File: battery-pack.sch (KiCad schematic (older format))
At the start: 54 parts, among them P1 CONN_01X02, U1 18650-PC8, U2 18650-PC8, U3 18650-PC8, U4 18650-PC8

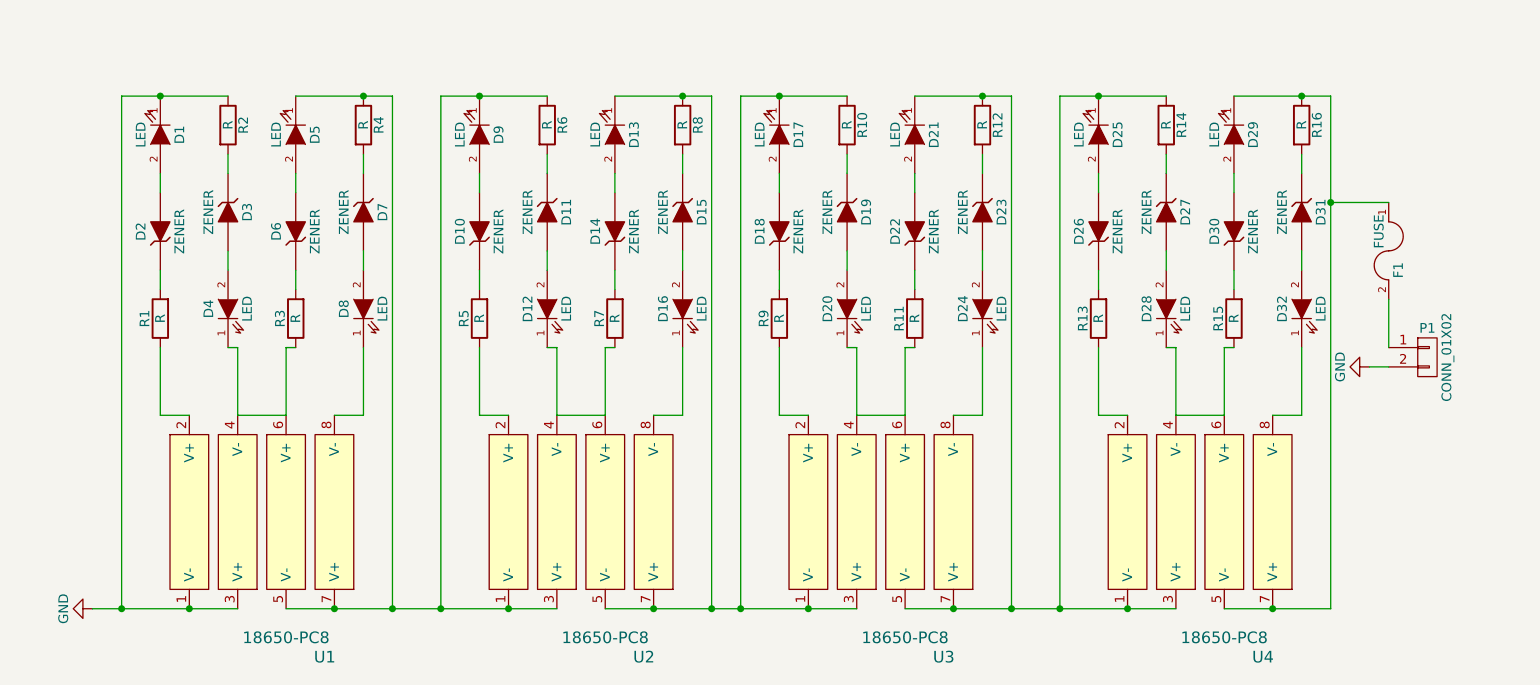
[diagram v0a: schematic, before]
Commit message: updated schematic
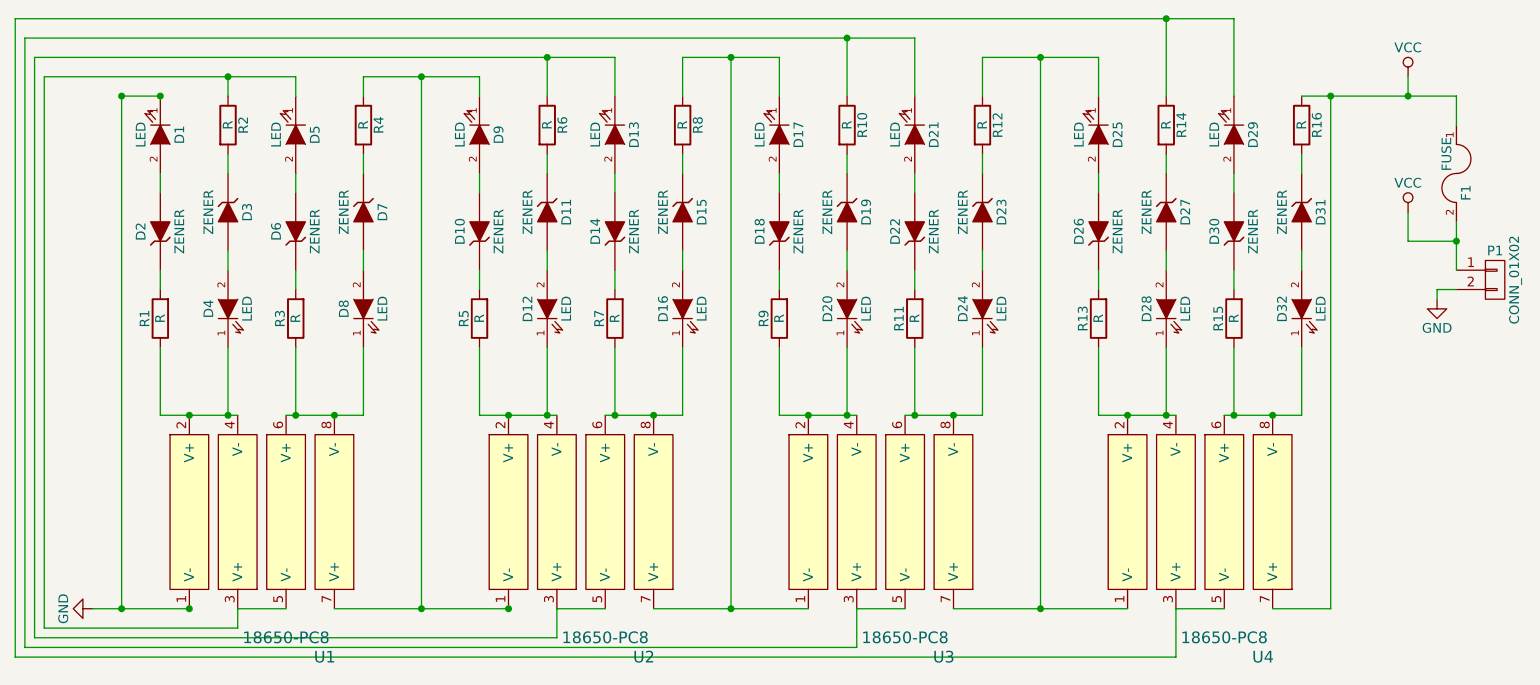
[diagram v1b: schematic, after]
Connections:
- net GND: no longer R2.1, U1.3 (V+)
- net at R1.1, U1.2 (V+): now also D4.1 (K), U1.4 (V-)
- net at R3.1, U1.6 (V+): now also D8.1 (K), U1.8 (V-); no longer D4.1 (K), U1.4 (V-)
- net at D9.1 (K), R4.1, U1.7 (V+)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: no longer D5.1 (K), R6.1, U1.5 (V-), U2.3 (V+)
- net at R5.1, U2.2 (V+): now also D12.1 (K), U2.4 (V-)
- net at R7.1, U2.6 (V+): now also D16.1 (K), U2.8 (V-); no longer D12.1 (K), U2.4 (V-)
- net at D17.1 (K), R8.1, U2.7 (V+)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: no longer D13.1 (K), R10.1, U2.5 (V-), U3.3 (V+)
- net at R9.1, U3.2 (V+): now also D20.1 (K), U3.4 (V-)
- net at R11.1, U3.6 (V+): now also D24.1 (K), U3.8 (V-); no longer D20.1 (K), U3.4 (V-)
- net at D25.1 (K), R12.1, U3.7 (V+)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: no longer D21.1 (K), R14.1, U3.5 (V-), U4.3 (V+)
- net at R13.1, U4.2 (V+): now also D28.1 (K), U4.4 (V-)
- net at R15.1, U4.6 (V+): now also D32.1 (K), U4.8 (V-); no longer D28.1 (K), U4.4 (V-)
- net VCC: now reaches F1.1, R16.1, U4.7 (V+)
- net VCC: now also F1.2, P1.1 (P1); no longer D29.1 (K), U4.5 (V-)
- new net: D5.1 (K), R2.1, U1.3 (V+), U1.5 (V-)
- new net: D13.1 (K), R6.1, U2.3 (V+), U2.5 (V-)
- new net: D21.1 (K), R10.1, U3.3 (V+), U3.5 (V-)
- new net: D29.1 (K), R14.1, U4.3 (V+), U4.5 (V-)
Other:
- moved on the sheet: F1, P1

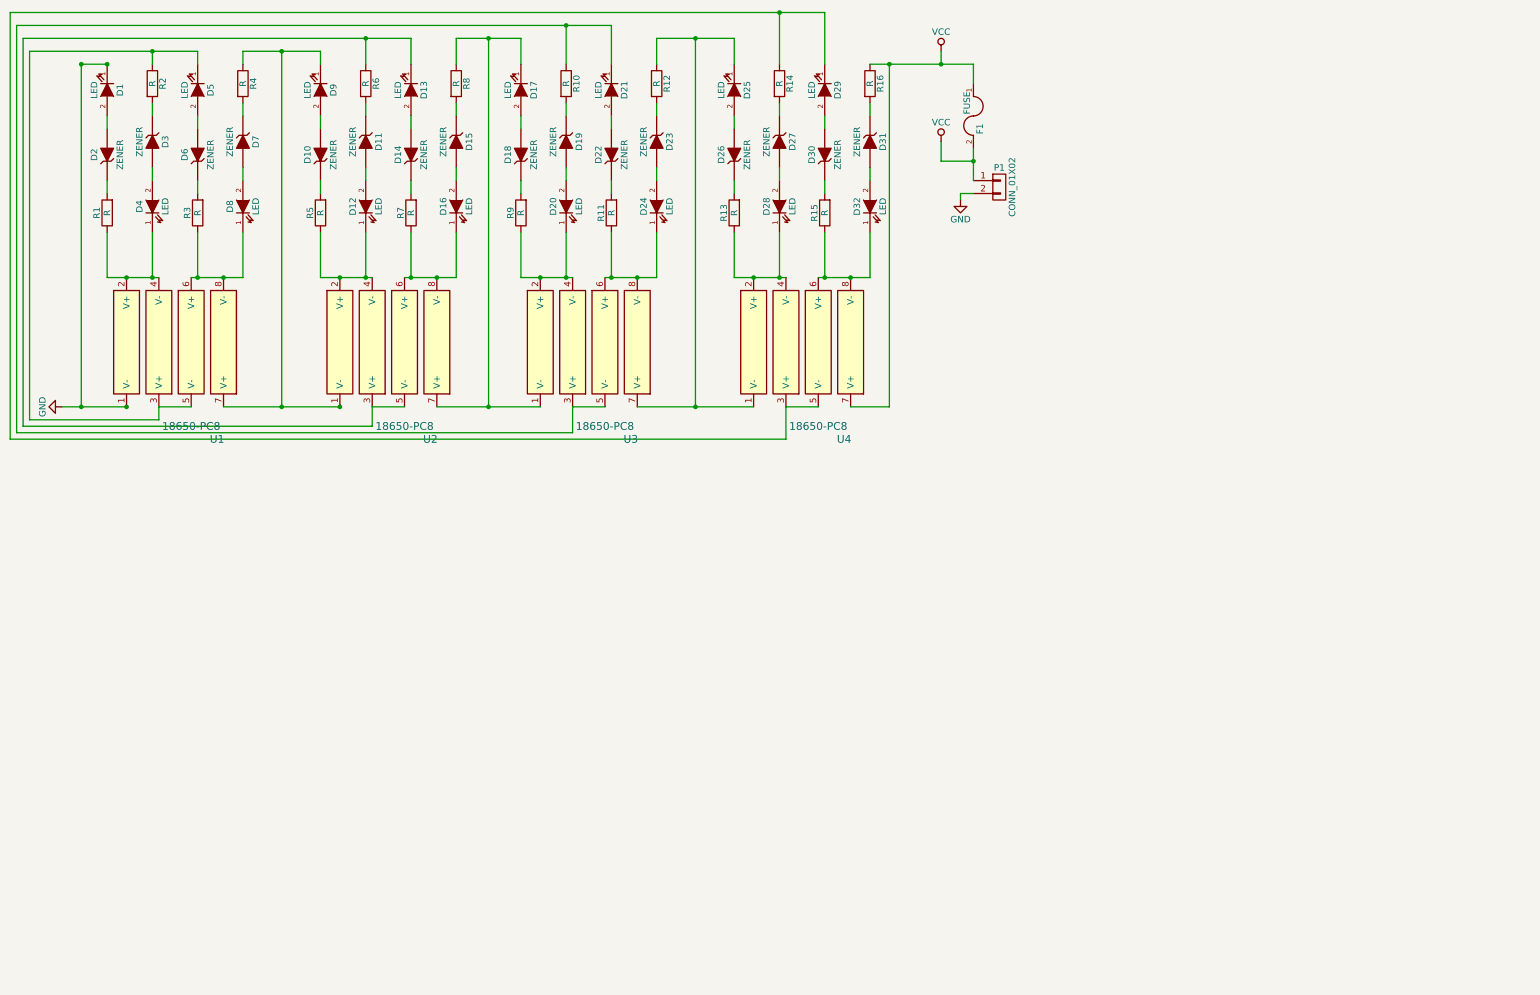
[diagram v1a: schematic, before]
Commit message: update
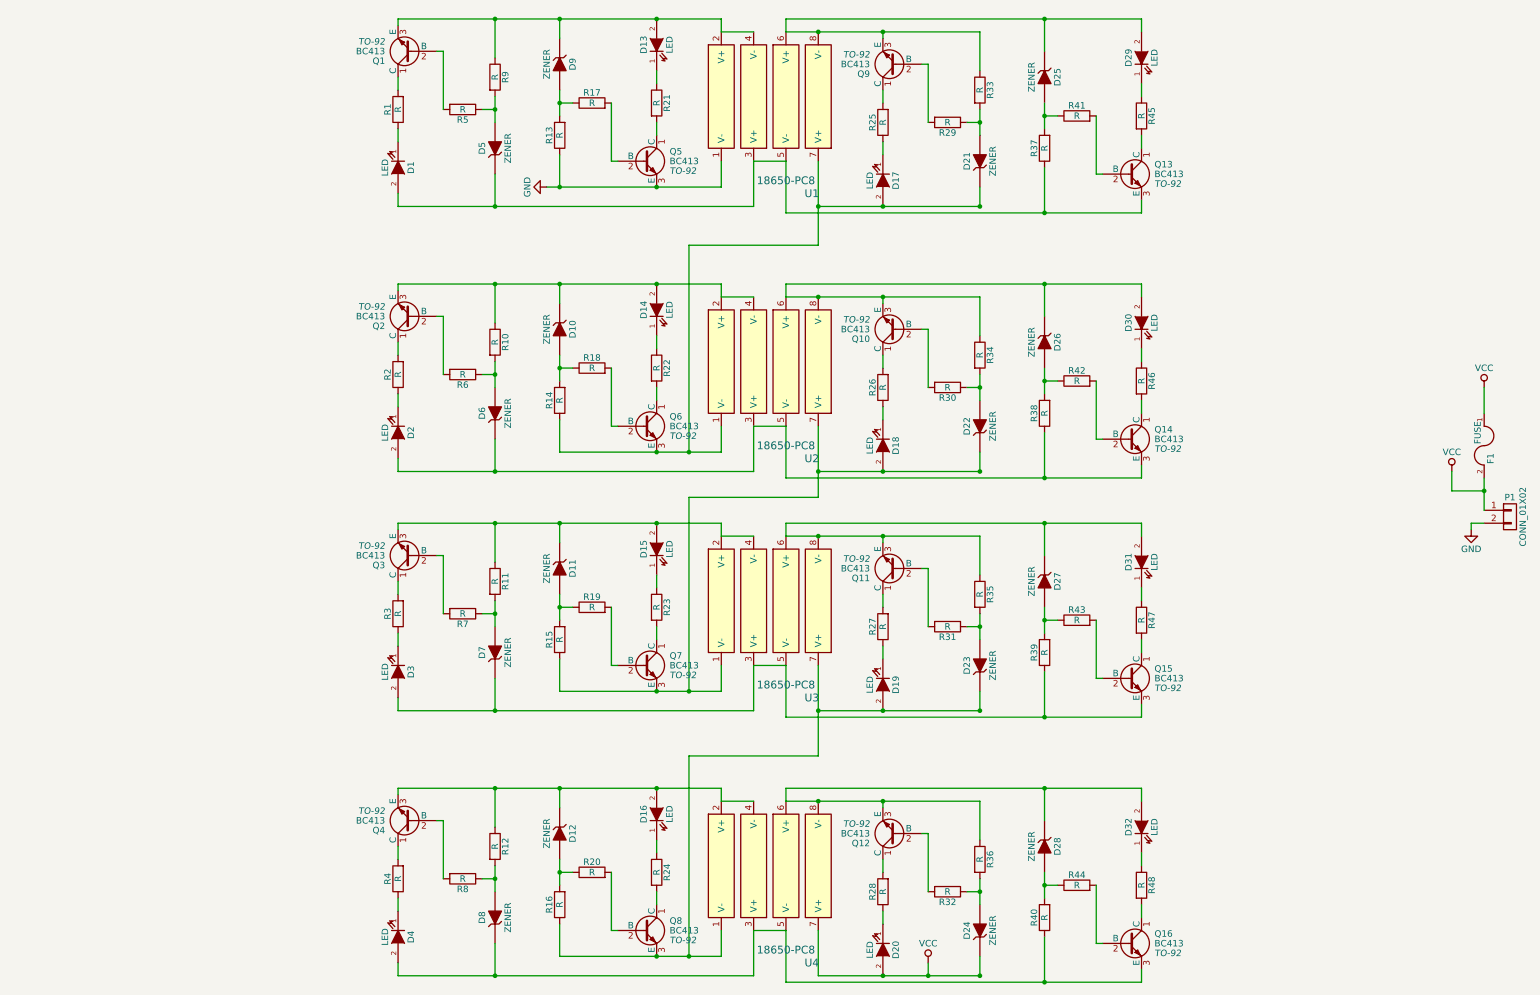
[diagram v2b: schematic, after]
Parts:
- removed D12, D21, D24, D25, D28, D5, D8, D9: LED, LEDs:LED-1206, symbol LED
- removed D14, D15, D18, D19, D2, D3, D30, D31: ZENER, LEDs:LED-1206, symbol ZENER
- added D12, D21, D24, D25, D28, D5, D8, D9: ZENER, LEDs:LED-1206, symbol ZENER
- added D14, D15, D18, D19, D2, D3, D30, D31: LED, LEDs:LED-1206, symbol LED
- added Q1, Q10, Q11, Q12, Q13, Q14, Q15, Q16, Q2, Q3, Q4, Q5, Q6, Q7, Q8, Q9: BC413, TO-92, symbol BC413
- added R17, R18, R19, R20, R21, R22, R23, R24, R25, R26, R27, R28, R29, R30, R31, R32, R33, R34, R35, R36, R37, R38, R39, R40, R41, R42, R43, R44, R45, R46, R47, R48: R, Resistors_SMD:R_1206, symbol R
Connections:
- net GND: now also R13.1, Q5.3 (E); no longer D1.1 (K)
- net VCC: now also D20.2 (A), D24.1 (K); no longer R16.1
- net at U1.2 (V+), U1.4 (V-): now also D13.2 (A), R9.1, D9.1 (K), Q1.3 (E); no longer D4.1 (K), R1.1
- net at U1.3 (V+), U1.5 (V-): now also D1.2 (A), D5.1 (K), Q13.3 (E), R37.1; no longer R2.1
- net at U1.6 (V+), U1.8 (V-): now also D29.2 (A), D25.1 (K), Q9.3 (E), R33.1; no longer R3.1
- net at U1.7 (V+), U2.1 (V-): now also D17.2 (A), R14.1, D21.1 (K), Q6.3 (E); no longer R4.1
- net at D4.2 (A): now also U4.3 (V+), U4.5 (V-), D8.1 (K), Q16.3 (E), R40.1
- net at R2.2: now also Q2.1 (C)
- net at R1.2: now also Q1.1 (C)
- net at D7.2 (A): now also R11.2, R7.1
- net at D7.1 (K): now also U3.3 (V+), U3.5 (V-), D3.2 (A), Q15.3 (E), R39.1; no longer R4.2
- net at D6.2 (A): now also R10.2, R6.1
- net at R3.2: now also Q3.1 (C); no longer D6.1 (K)
- net at U2.2 (V+), U2.4 (V-): now also D10.1 (K), R10.1, D14.2 (A), Q2.3 (E); no longer R5.1
- net at U2.3 (V+), U2.5 (V-): now also D6.1 (K), D2.2 (A), Q14.3 (E), R38.1; no longer D13.1 (K), R6.1
- net at U2.6 (V+), U2.8 (V-): now also D26.1 (K), D30.2 (A), Q10.3 (E), R34.1; no longer D16.1 (K), R7.1
- net at U2.7 (V+), U3.1 (V-): now also D22.1 (K), R15.1, D18.2 (A), Q7.3 (E); no longer D17.1 (K), R8.1
- net at D11.2 (A): now also R15.2, R19.1
- net at D11.1 (K): now also R11.1, U3.2 (V+), U3.4 (V-), D15.2 (A), Q3.3 (E); no longer R6.2
- net at D10.2 (A): now also R14.2, R18.1
- net at R5.2: now also Q1.2 (B); no longer D10.1 (K)
- net at D16.2 (A): now also R12.1, U4.2 (V+), U4.4 (V-), D12.1 (K), Q4.3 (E)
- net at R8.2: now also Q4.2 (B)
- net at R7.2: now also Q3.2 (B)
- net at U3.6 (V+), U3.8 (V-): now also D27.1 (K), D31.2 (A), Q11.3 (E), R35.1; no longer R11.1
- net at U3.7 (V+), U4.1 (V-): now also D23.1 (K), R16.1, D19.2 (A), Q8.3 (E); no longer R12.1
- net at R9.2: now also R5.1, D5.2 (A)
- net at D23.2 (A): now also R31.1, R35.2
- net at R12.2: now also R8.1, D8.2 (A); no longer D23.1 (K)
- net at D22.2 (A): now also R30.1, R34.2
- net at U4.6 (V+), U4.8 (V-): now also D32.2 (A), D28.1 (K), Q12.3 (E), R36.1; no longer D32.1 (K), R15.1
- net at D27.2 (A): now also R39.2, R43.1
- net at D26.2 (A): now also R38.2, R42.1
- net at R13.2: now also D9.2 (A), R17.1; no longer D26.1 (K)
- net at R16.2: now also D12.2 (A), R20.1
- new net: Q7.1 (C), R23.2
- new net: Q7.2 (B), R19.2
- new net: D15.1 (K), R23.1
- new net: D3.1 (K), R3.1
- new net: Q11.1 (C), R27.2
- new net: Q11.2 (B), R31.2
- new net: D19.1 (K), R27.1
- new net: Q15.1 (C), R47.2
- new net: Q15.2 (B), R43.2
- new net: D31.1 (K), R47.1
- new net: Q8.1 (C), R24.2
- new net: Q8.2 (B), R20.2
- new net: D16.1 (K), R24.1
- new net: Q4.1 (C), R4.2
- new net: D4.1 (K), R4.1
- new net: D24.2 (A), R32.1, R36.2
- new net: Q12.1 (C), R28.2
- new net: Q12.2 (B), R32.2
- new net: D20.1 (K), R28.1
- new net: D28.2 (A), R40.2, R44.1
- new net: Q16.1 (C), R48.2
- new net: Q16.2 (B), R44.2
- new net: D32.1 (K), R48.1
- new net: Q5.1 (C), R21.2
- new net: Q5.2 (B), R17.2
- new net: D13.1 (K), R21.1
- new net: D1.1 (K), R1.1
- new net: D21.2 (A), R29.1, R33.2
- new net: Q9.1 (C), R25.2
- new net: Q9.2 (B), R29.2
- new net: D17.1 (K), R25.1
- new net: D25.2 (A), R37.2, R41.1
- new net: Q13.1 (C), R45.2
- new net: Q13.2 (B), R41.2
- new net: D29.1 (K), R45.1
- new net: Q6.1 (C), R22.2
- new net: Q6.2 (B), R18.2
- new net: D14.1 (K), R22.1
- new net: Q2.2 (B), R6.2
- new net: D2.1 (K), R2.1
- new net: Q10.1 (C), R26.2
- new net: Q10.2 (B), R30.2
- new net: D18.1 (K), R26.1
- new net: Q14.1 (C), R46.2
- new net: Q14.2 (B), R42.2
- new net: D30.1 (K), R46.1
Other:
- moved on the sheet: F1, P1

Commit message: update
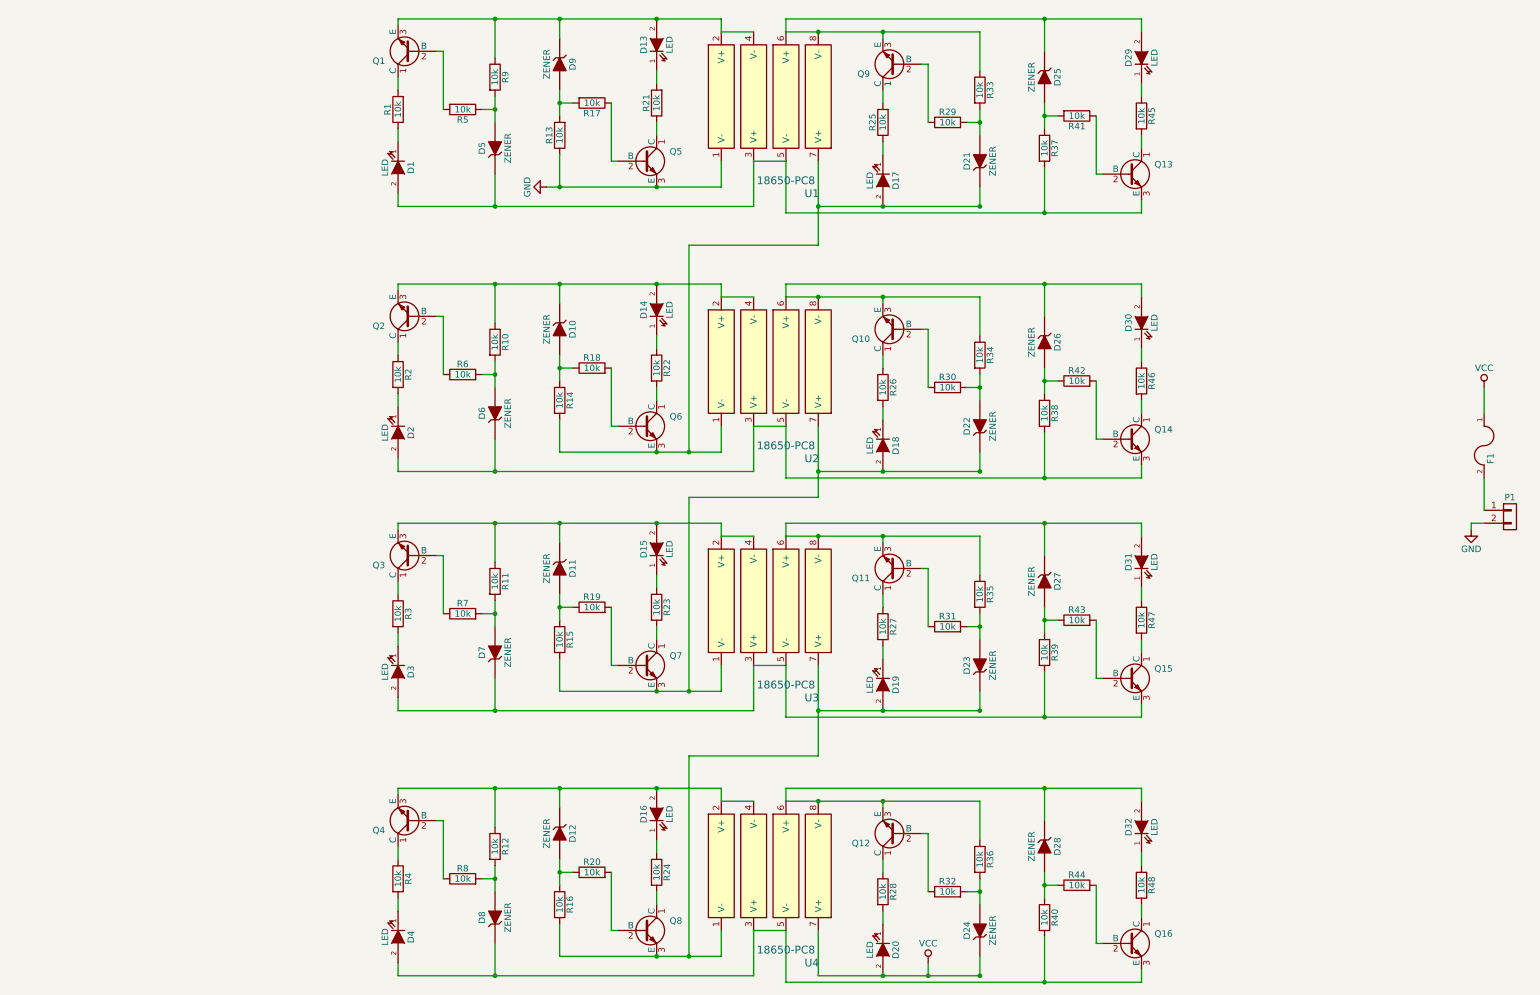
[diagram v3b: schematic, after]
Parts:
- D1, D13, D14, D15, D16, D17, D18, D19, D2, D20, D29, D3, D30, D31, D32, D4: footprint LEDs:LED-1206 -> LEDs:LED_0805
- D10, D11, D12, D21, D22, D23, D24, D25, D26, D27, D28, D6, D7, D8, D9: footprint LEDs:LED-1206 -> TO_SOT_Packages_SMD:SOT-23
- D5: footprint LEDs:LED-1206 -> Diodes_ThroughHole:Diode_P600_Horizontal
- F1: value FUSE -> 01000057Z; footprint battery-pack:fuse-holder-BK6010 -> battery-pack:ATC_FUSE
- Q1, Q10, Q11, Q12, Q13, Q14, Q15, Q16, Q2, Q3, Q4, Q5, Q6, Q7, Q8, Q9: value BC413 -> MMBT3904LT1G; footprint TO-92 -> TO_SOT_Packages_SMD:SOT-23
- R1, R10, R11, R12, R13, R14, R15, R16, R17, R18, R19, R2, R20, R21, R22, R23, R24, R25, R26, R27, R28, R29, R3, R30, R31, R32, R33, R34, R35, R36, R37, R38, R39, R4, R40, R41, R42, R43, R44, R45, R46, R47, R48, R5, R6, R7, R8, R9: value R -> 10k; footprint Resistors_SMD:R_1206 -> Resistors_SMD:R_0805
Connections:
- net VCC: no longer F1.2, P1.1 (P1)
- net at D18.2 (A), D22.1 (K), Q7.3 (E)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: now also R15.2; no longer R15.1
- net at D3.2 (A), D7.1 (K), Q15.3 (E)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: now also R39.2; no longer R39.1
- net at D19.2 (A), D23.1 (K), Q8.3 (E)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: now also R16.2; no longer R16.1
- net at D11.2 (A), R19.1: now also R15.1; no longer R15.2
- net at D7.2 (A), R11.2: now also R7.2; no longer R7.1
- net at R3.2: now also D3.1 (K); no longer Q3.1 (C)
- net at Q3.2 (B): now also R7.1; no longer R7.2
- net at R3.1: now also Q3.1 (C); no longer D3.1 (K)
- net at D23.2 (A), R35.2: now also R31.2; no longer R31.1
- net at R27.2: now also D19.1 (K); no longer Q11.1 (C)
- net at Q11.2 (B): now also R31.1; no longer R31.2
- net at R27.1: now also Q11.1 (C); no longer D19.1 (K)
- net at D27.2 (A), R43.1: now also R39.1; no longer R39.2
- net at D4.2 (A), D8.1 (K), Q16.3 (E)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: now also R40.2; no longer R40.1
- net at D12.2 (A), R20.1: now also R16.1; no longer R16.2
- net at D8.2 (A), R12.2: now also R8.2; no longer R8.1
- net at R4.2: now also D4.1 (K); no longer Q4.1 (C)
- net at Q4.2 (B): now also R8.1; no longer R8.2
- net at R4.1: now also Q4.1 (C); no longer D4.1 (K)
- net at D24.2 (A), R36.2: now also R32.2; no longer R32.1
- net at R28.2: now also D20.1 (K); no longer Q12.1 (C)
- net at Q12.2 (B): now also R32.1; no longer R32.2
- net at R28.1: now also Q12.1 (C); no longer D20.1 (K)
- net at D28.2 (A), R44.1: now also R40.1; no longer R40.2
- net at D1.2 (A), D5.1 (K), Q13.3 (E)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: now also R37.2; no longer R37.1
- net at D17.2 (A), D21.1 (K), Q6.3 (E)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: now also R14.2; no longer R14.1
- net at D9.2 (A), R13.2: now also R17.2; no longer R17.1
- net at R21.2: now also D13.1 (K); no longer Q5.1 (C)
- net at Q5.2 (B): now also R17.1; no longer R17.2
- net at R21.1: now also Q5.1 (C); no longer D13.1 (K)
- net at D21.2 (A), R33.2: now also R29.2; no longer R29.1
- net at Q9.2 (B): now also R29.1; no longer R29.2
- net at R41.2: now also D25.2 (A), R37.1; no longer Q13.2 (B)
- net at D2.2 (A), D6.1 (K), Q14.3 (E)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: now also R38.2; no longer R38.1
- net at D10.2 (A), R18.1: now also R14.1; no longer R14.2
- net at D6.2 (A), R10.2: now also R6.2; no longer R6.1
- net at R2.2: now also D2.1 (K); no longer Q2.1 (C)
- net at Q2.2 (B): now also R6.1; no longer R6.2
- net at R2.1: now also Q2.1 (C); no longer D2.1 (K)
- net at D22.2 (A), R34.2: now also R30.2; no longer R30.1
- net at R26.2: now also D18.1 (K); no longer Q10.1 (C)
- net at Q10.2 (B): now also R30.1; no longer R30.2
- net at R26.1: now also Q10.1 (C); no longer D18.1 (K)
- net at D26.2 (A), R42.1: now also R38.1; no longer R38.2
- new net: F1.2, P1.1 (P1)
- new net: Q13.2 (B), R41.1
